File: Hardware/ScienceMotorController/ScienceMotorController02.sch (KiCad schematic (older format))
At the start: 5 parts, among them U1 TM4C129E_Launchpad

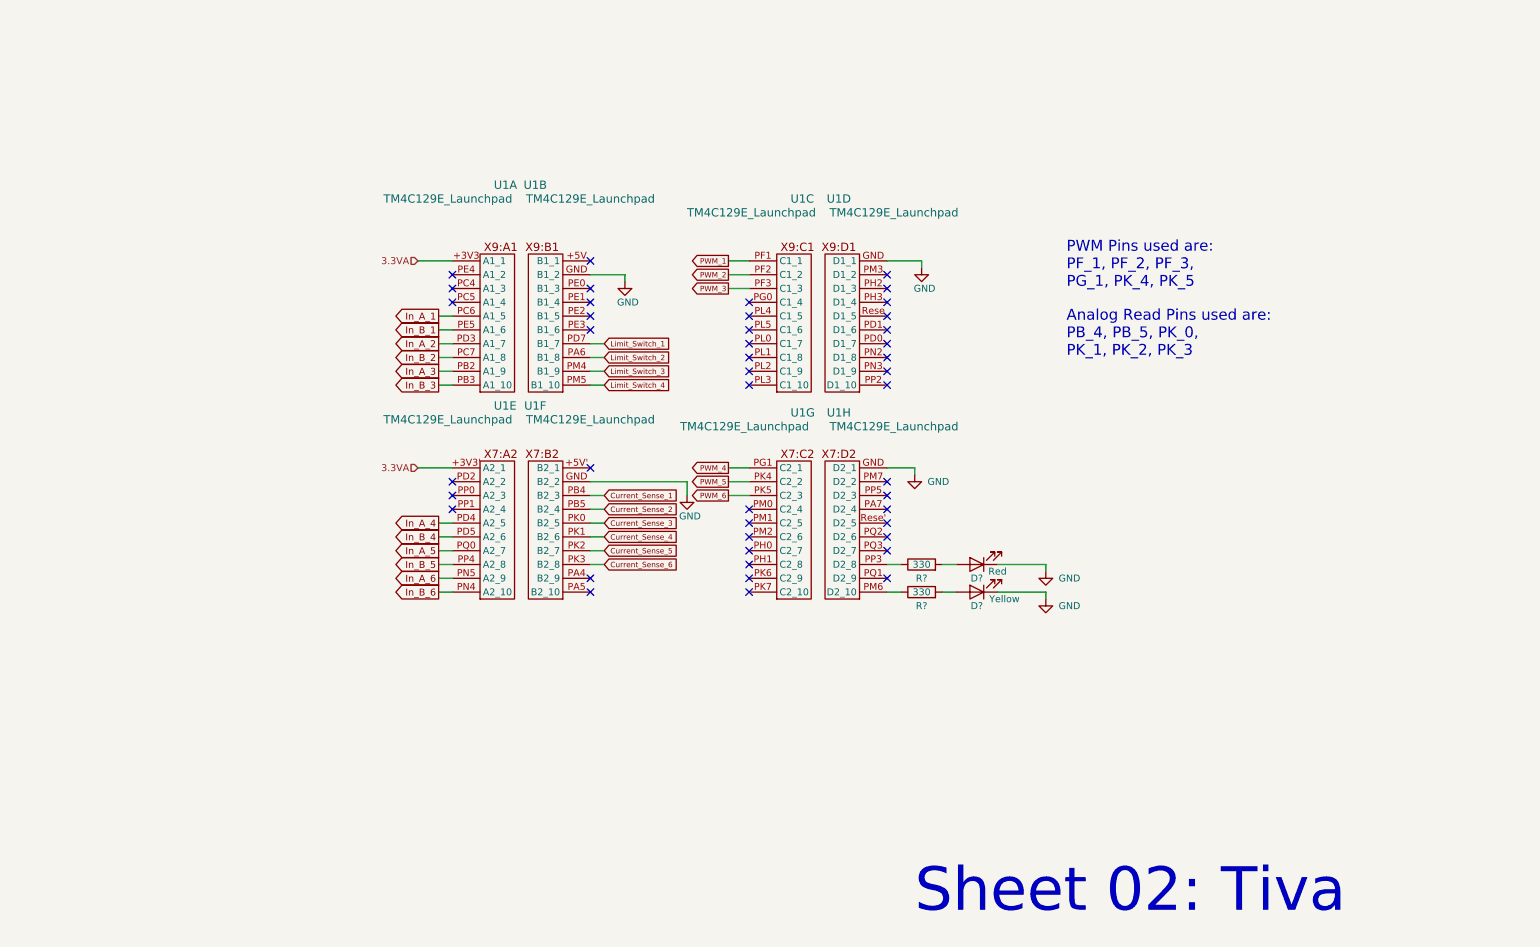
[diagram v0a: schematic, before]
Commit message: fixed hierarchical
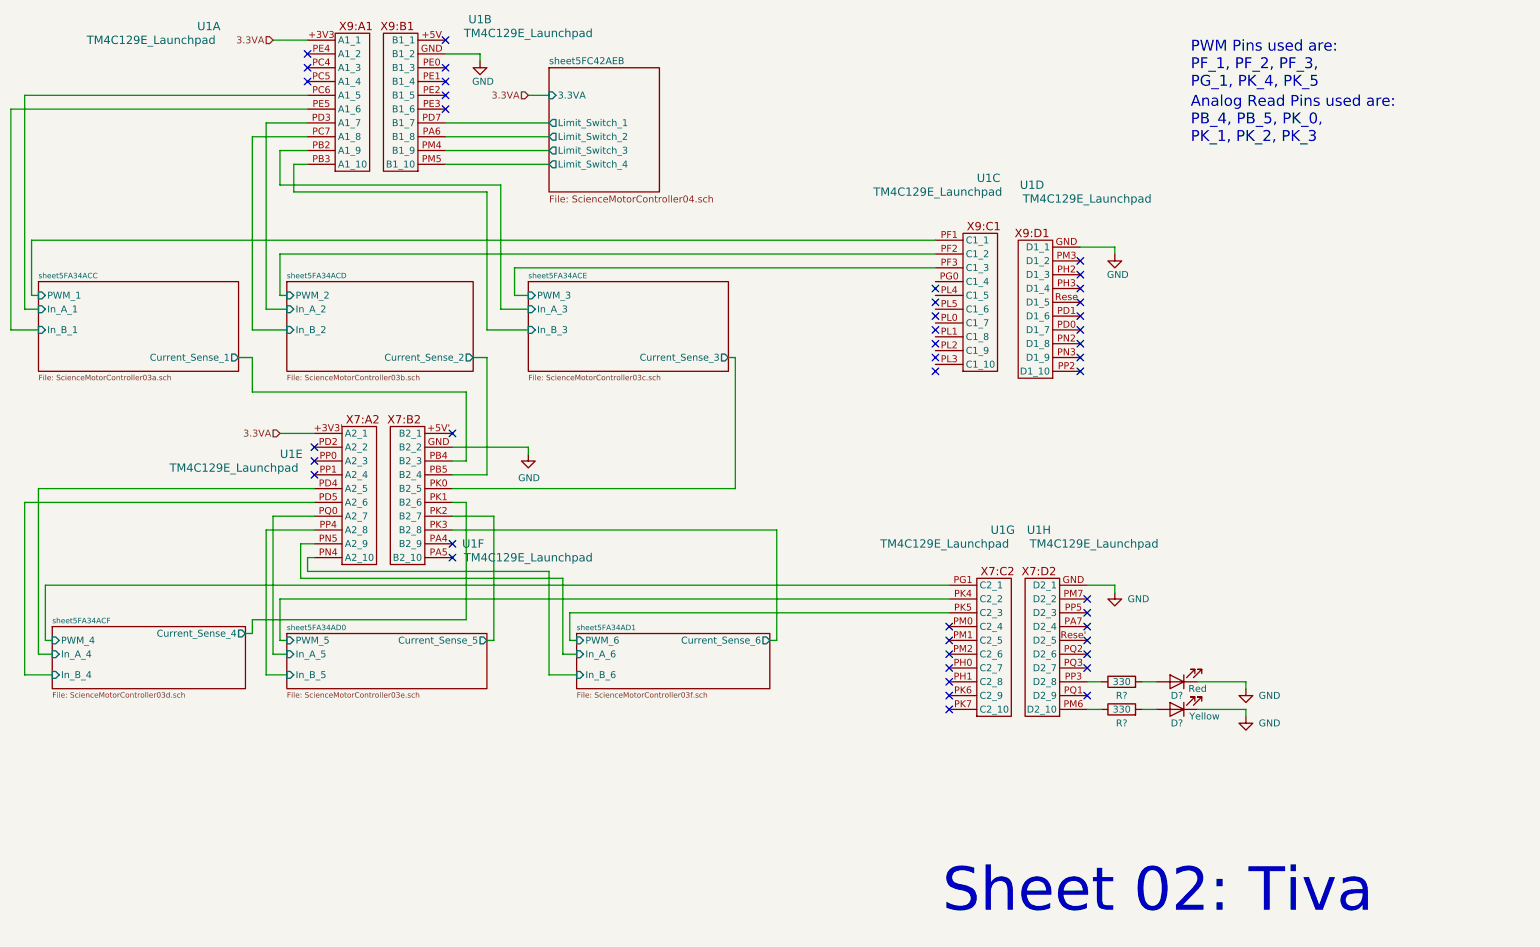
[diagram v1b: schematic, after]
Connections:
- net Current_Sense_1 renamed sheet5FA34ACC/Current_Sense_1
- net Current_Sense_2 renamed sheet5FA34ACD/Current_Sense_2
- net Current_Sense_3 renamed sheet5FA34ACE/Current_Sense_3
- net Current_Sense_4 renamed sheet5FA34ACF/Current_Sense_4
- net Current_Sense_5 renamed sheet5FA34AD0/Current_Sense_5
- net Current_Sense_6 renamed sheet5FA34AD1/Current_Sense_6
- net In_A_1 renamed sheet5FA34ACC/In_A_1
- net In_A_2 renamed sheet5FA34ACD/In_A_2
- net In_A_3 renamed sheet5FA34ACE/In_A_3
- net In_A_4 renamed sheet5FA34ACF/In_A_4
- net In_A_5 renamed sheet5FA34AD0/In_A_5
- net In_A_6 renamed sheet5FA34AD1/In_A_6
- net In_B_1 renamed sheet5FA34ACC/In_B_1
- net In_B_2 renamed sheet5FA34ACD/In_B_2
- net In_B_3 renamed sheet5FA34ACE/In_B_3
- net In_B_4 renamed sheet5FA34ACF/In_B_4
- net In_B_5 renamed sheet5FA34AD0/In_B_5
- net In_B_6 renamed sheet5FA34AD1/In_B_6
- net Limit_Switch_1 renamed sheet5FC42AEB/Limit_Switch_1
- net Limit_Switch_2 renamed sheet5FC42AEB/Limit_Switch_2
- net Limit_Switch_3 renamed sheet5FC42AEB/Limit_Switch_3
- net Limit_Switch_4 renamed sheet5FC42AEB/Limit_Switch_4
- net PWM_1 renamed sheet5FA34ACC/PWM_1
- net PWM_2 renamed sheet5FA34ACD/PWM_2
- net PWM_3 renamed sheet5FA34ACE/PWM_3
- net PWM_4 renamed sheet5FA34ACF/PWM_4
- net PWM_5 renamed sheet5FA34AD0/PWM_5
- net PWM_6 renamed sheet5FA34AD1/PWM_6
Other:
- moved on the sheet: D?, R?, U1A, U1B, U1C, U1D, U1E, U1F, U1G, U1H
